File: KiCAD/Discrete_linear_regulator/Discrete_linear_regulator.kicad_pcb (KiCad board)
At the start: 4 copper layers, 40.1 x 36 mm, 40 parts, among them J1 Conn_01x06, Q1 PZT2222AT3G, Q10 BC857, Q11 BC857, Q2 BC857, Q3 BC857, Q4 PZT2222AT3G, Q5 PZT2907AT3G, Q8 PZT2907AT3G, U1 LM4562

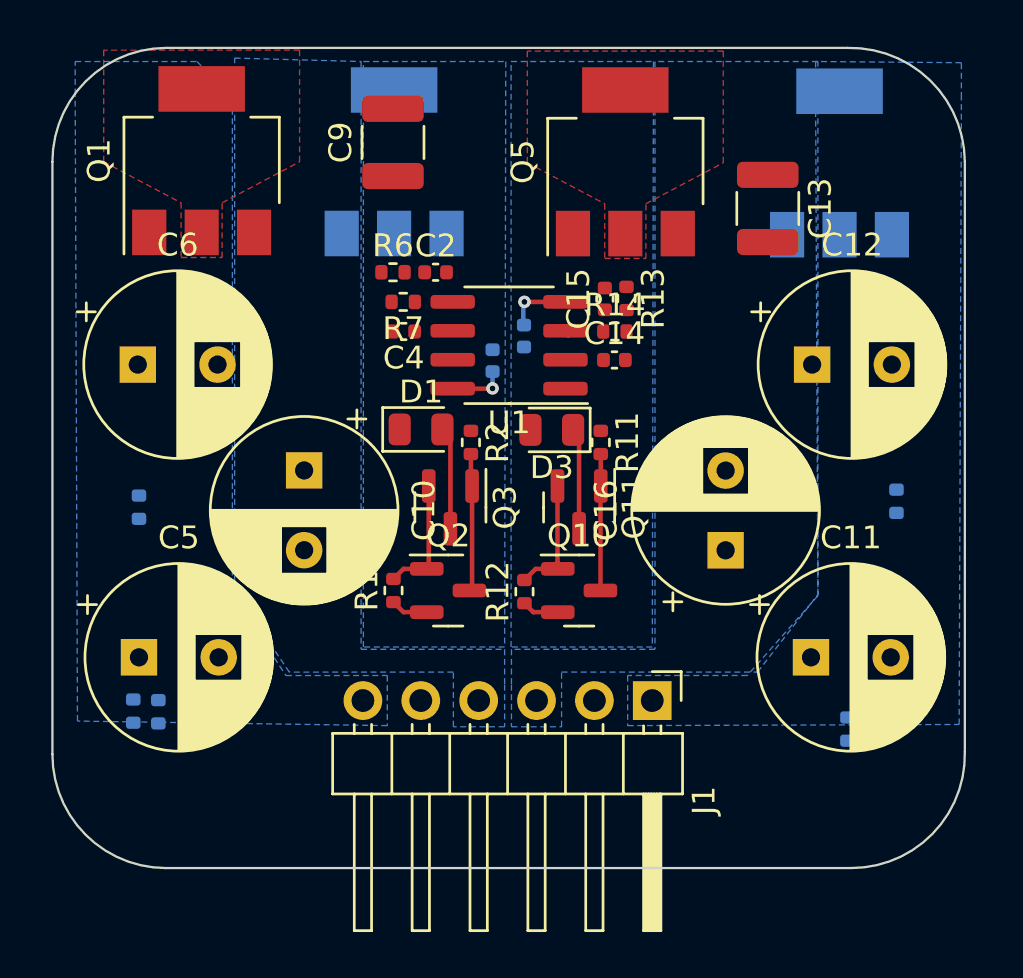
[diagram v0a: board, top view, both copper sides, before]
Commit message: update linear
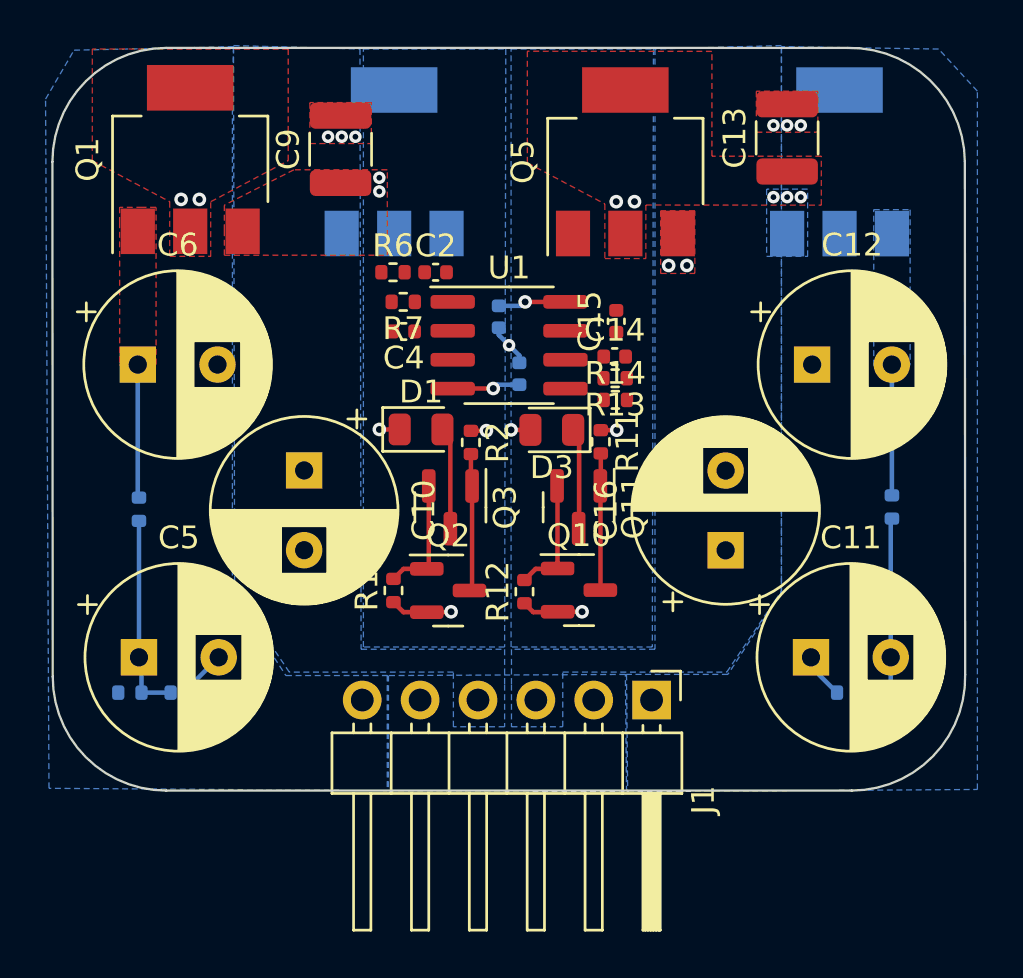
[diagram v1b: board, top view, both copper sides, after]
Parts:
- Q10, Q11: value BC857 -> BC847
- R1, R12: value 780R -> 820R
- moved R13 3.54 mm to (153.8, 95.0), turned to 180 degrees
- moved C13 3.21 mm to (161.3, 84.5), turned to 90 degrees
- moved R14 3.00 mm to (153.8, 96.0)
- moved C9 2.32 mm to (141.7, 85.0)
- moved R8 2.16 mm to (166.3, 108.8), turned to 180 degrees
- moved C1 1.94 mm to (148.6, 92.3), turned to -90 degrees
- moved C3 1.67 mm to (149.5, 94.8), turned to -90 degrees
- moved R9 1.60 mm to (164.0, 108.8), turned to 0 degrees
- moved R5 1.34 mm to (134.8, 108.8), turned to 180 degrees
- moved C15 1.10 mm to (153.8, 92.5)
- moved R4 0.82 mm to (132.4, 108.8), turned to 0 degrees
- moved Q1 0.50 mm to (135.1, 85.4)
- moved R10 0.32 mm to (165.9, 100.7)
- moved C14 0.15 mm to (153.7, 94.0)
- moved R3 0.09 mm to (132.8, 100.8)
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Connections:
- C15 pad 1: Net-(U1A-+) -> Net-(U1B-+)
- C2 pad 1: Net-(U1B-+) -> Net-(U1A-+)
- R13 pad 2: Net-(U1A-+) -> Net-(U1B-+)
- R14 pad 1: Net-(U1A-+) -> Net-(U1B-+)
- R6 pad 2: Net-(U1B-+) -> Net-(U1A-+)
- R7 pad 1: Net-(U1B-+) -> Net-(U1A-+)
- U1 pad 1: Net-(C15-Pad2) -> Net-(C2-Pad2)
- U1 pad 2: Net-(D3-K) -> Net-(D1-A)
- U1 pad 6: Net-(D1-A) -> Net-(D3-K)
- U1 pad 7: Net-(C2-Pad2) -> Net-(C15-Pad2)
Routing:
- net GND: track 0.07 -> 9.66 mm, vias 0 -> 11
- net Net-(C11-Pad2): track 0.00 -> 9.04 mm
- net Net-(C5-Pad1): track 0.00 -> 8.87 mm
- net Net-(C6-Pad1): track 0.00 -> 6.58 mm
- net Net-(C12-Pad2): track 0.00 -> 5.82 mm
- net V+: track 4.27 -> 5.72 mm, vias 1 -> 4
- net V-: track 4.54 -> 5.78 mm, vias 1 -> 7
- net Net-(U1A-+): track 1.08 -> 0.00 mm
- net -12V: vias 0 -> 2
- net +15V: vias 0 -> 2
- added copper zone on F.Cu, net -12V
- added copper zone on B.Cu, net GND
- added copper zone on F.Cu, net GND
- added copper zone on In1.Cu, net GND
- added copper zone on In2.Cu, net GND
- added copper zone on B.Cu, net Net-(C12-Pad2)
- added copper zone on F.Cu, net Net-(C6-Pad1)
- added copper zone on F.Cu, net V+
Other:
- board size 40.1 x 36 mm -> 40.1 x 32.6 mm

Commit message: update linear and gerbers
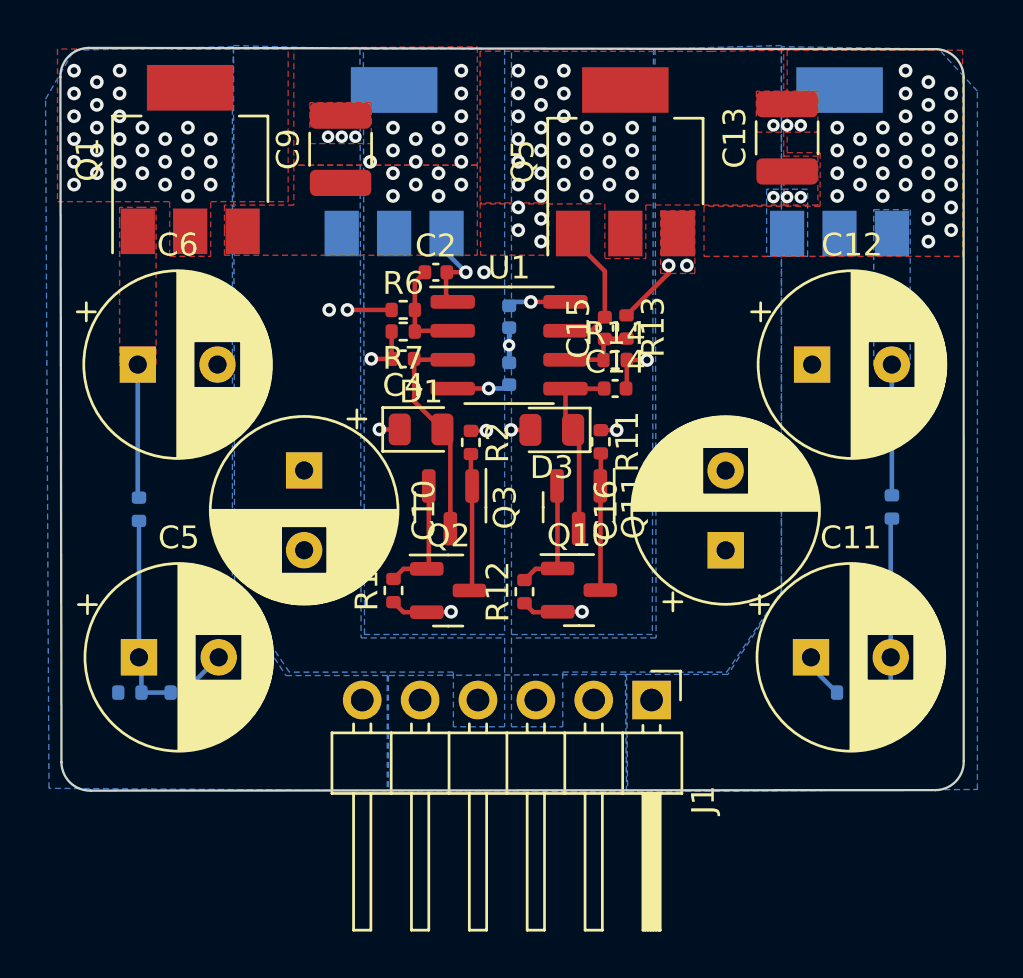
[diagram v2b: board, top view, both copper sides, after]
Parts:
- moved R13 2.30 mm to (154.2, 92.8), turned to -90 degrees
- moved R14 1.75 mm to (153.8, 94.2)
- moved R6 1.71 mm to (144.4, 92.0)
- moved C14 1.40 mm to (153.8, 95.5)
- moved R7 1.30 mm to (144.4, 93.0)
- moved C4 1.20 mm to (144.4, 94.2)
- moved C15 0.58 mm to (153.3, 92.8)
- moved C1 0.46 mm to (149.1, 92.3)
- moved C3 0.44 mm to (149.1, 94.8)
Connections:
- C15 pad 1: Net-(U1B-+) -> Net-(U1B--)
- C2 pad 1: Net-(U1A-+) -> Net-(U1A--)
- R13 pad 2: Net-(U1B-+) -> Net-(U1B--)
- R14 pad 1: Net-(U1B-+) -> Net-(U1B--)
- R6 pad 2: Net-(U1A-+) -> Net-(U1A--)
- R7 pad 1: Net-(U1A-+) -> Net-(U1A--)
- U1 pad 2: Net-(D1-A) -> Net-(U1A--)
- U1 pad 3: Net-(U1A-+) -> Net-(D1-A)
- U1 pad 5: Net-(U1B-+) -> Net-(D3-K)
- U1 pad 6: Net-(D3-K) -> Net-(U1B--)
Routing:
- net Net-(C15-Pad2): track 0.00 -> 6.23 mm
- net Net-(D1-A): track 4.94 -> 9.82 mm
- net Net-(U1A--): track 0.00 -> 4.46 mm
- net Net-(C2-Pad2): track 0.00 -> 4.31 mm, vias 0 -> 1
- net GND: track 9.66 -> 13.4 mm, vias 11 -> 15
- net Net-(U1B--): track 0.00 -> 3.58 mm
- net Net-(D3-K): track 4.59 -> 8.10 mm
- net -12V: track 0.00 -> 2.96 mm
- net +12V: track 0.00 -> 1.94 mm, vias 0 -> 1
- net V-: track 5.78 -> 5.25 mm, vias 7 -> 38
- net V+: track 5.72 -> 5.51 mm, vias 4 -> 20
- net -15V: vias 0 -> 32
- net +15V: vias 2 -> 30
- added copper zone on F.Cu, net -15V
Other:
- board size 40.1 x 32.6 mm -> 39.7 x 32.6 mm
- board text added: "JLCJLCJLCJLC"
